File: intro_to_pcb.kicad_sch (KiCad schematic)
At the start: 0 parts

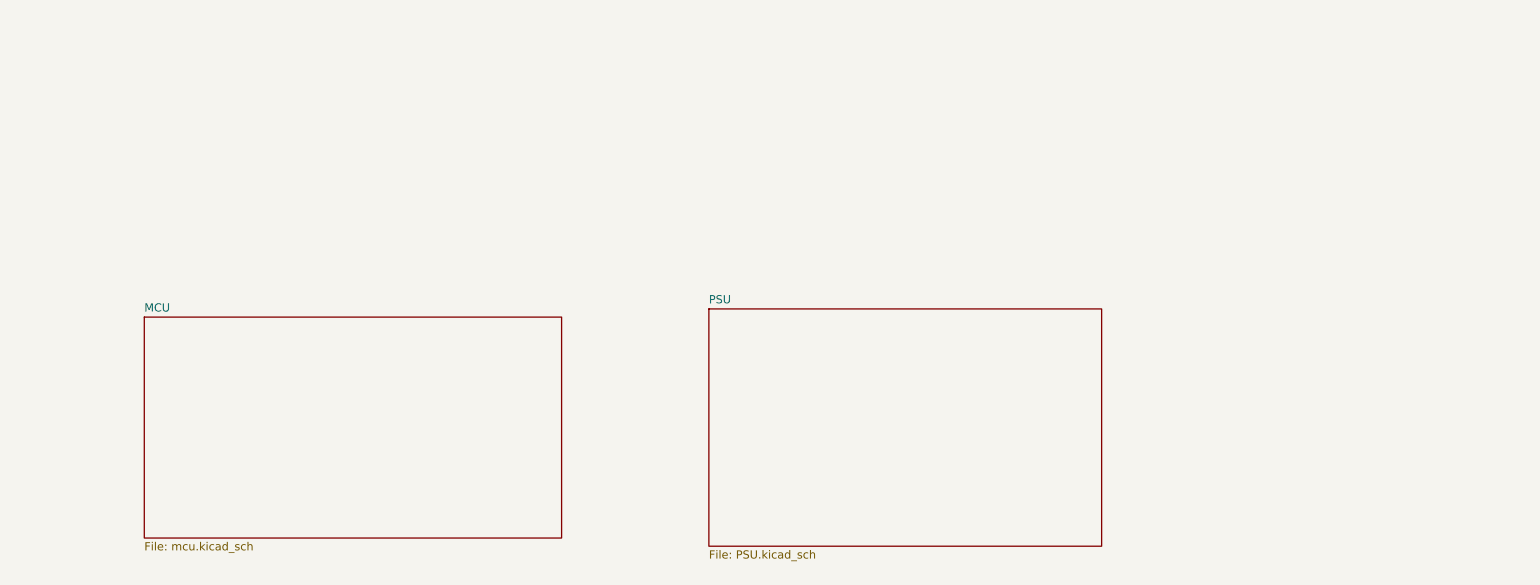
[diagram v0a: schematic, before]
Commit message: Fixing git
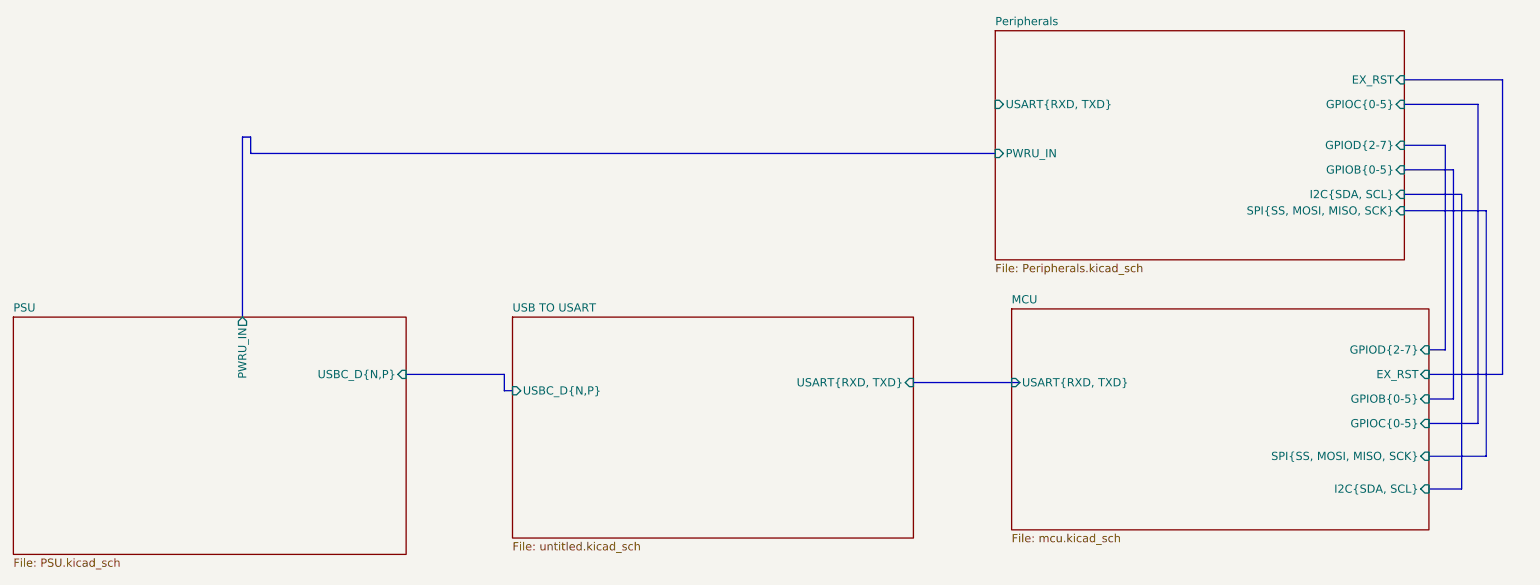
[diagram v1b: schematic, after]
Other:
- added sheet Peripherals (Peripherals.kicad_sch)
- added sheet USB TO USART (untitled.kicad_sch)
- sheet MCU ports: added EX_RST, GPIOB{0-5}, GPIOC{0-5}, GPIOD{2-7}, I2C{SDA, SCL}, SPI{SS, MOSI, MISO, SCK}, USART{RXD, TXD}; removed none
- sheet PSU ports: added PWRU_IN, USBC_D{N,P}; removed none
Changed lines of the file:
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@@
 (kicad_sch (version 20230121) (generator eeschema)
   (paper "A4")
-  (sheet (at 54.61 99.06) (size 64.77 34.29) (fields_autoplaced)
+  (bus (pts (xy 110.49 110.49) (xy 111.76 110.49))
+    (stroke (width 0) (type default))
+  )
+  (bus (pts (xy 71.12 71.12) (xy 69.85 71.12))
+    (stroke (width 0) (type default))
+  )
+  (bus (pts (xy 262.89 82.55) (xy 250.19 82.55))
+    (stroke (width 0) (type default))
+  )
+  (bus (pts (xy 257.81 111.76) (xy 254 111.76))
+    (stroke (width 0) (type default))
+  )
+  (bus (pts (xy 250.19 76.2) (xy 257.81 76.2))
+    (stroke (width 0) (type default))
+  )
+  (bus (pts (xy 265.43 107.95) (xy 254 107.95))
+    (stroke (width 0) (type default))
+  )
+  (bus (pts (xy 257.81 76.2) (xy 257.81 111.76))
+    (stroke (width 0) (type default))
+  )
+  (bus (pts (xy 110.49 107.95) (xy 110.49 110.49))
+    (stroke (width 0) (type default))
+  )
+  (bus (pts (xy 256.54 72.39) (xy 256.54 104.14))
+    (stroke (width 0) (type default))
+  )
+  (bus (pts (xy 261.62 115.57) (xy 254 115.57))
+    (stroke (width 0) (type default))
+  )
+  (bus (pts (xy 173.99 109.22) (xy 190.5 109.22))
+    (stroke (width 0) (type default))
+  )
+  (bus (pts (xy 254 125.73) (xy 259.08 125.73))
+    (stroke (width 0) (type default))
+  )
+  (bus (pts (xy 71.12 71.12) (xy 71.12 73.66))
+    (stroke (width 0) (type default))
+  )
+  (bus (pts (xy 95.25 107.95) (xy 110.49 107.95))
+    (stroke (width 0) (type default))
+  )
+  (bus (pts (xy 265.43 62.23) (xy 265.43 107.95))
+    (stroke (width 0) (type default))
+  )
+  (bus (pts (xy 262.89 120.65) (xy 262.89 82.55))
+    (stroke (width 0) (type default))
+  )
+  (bus (pts (xy 259.08 80.01) (xy 250.19 80.01))
+    (stroke (width 0) (type default))
+  )
+  (bus (pts (xy 250.19 62.23) (xy 265.43 62.23))
+    (stroke (width 0) (type default))
+  )
+  (bus (pts (xy 250.19 72.39) (xy 256.54 72.39))
+    (stroke (width 0) (type default))
+  )
+  (bus (pts (xy 259.08 125.73) (xy 259.08 80.01))
+    (stroke (width 0) (type default))
+  )
+  (bus (pts (xy 261.62 66.04) (xy 261.62 115.57))
+    (stroke (width 0) (type default))
+  )
+  (bus (pts (xy 69.85 71.12) (xy 69.85 99.06))
+    (stroke (width 0) (type default))
+  )
+  (bus (pts (xy 256.54 104.14) (xy 254 104.14))
+    (stroke (width 0) (type default))
+  )
+  (bus (pts (xy 71.12 73.66) (xy 186.69 73.66))
+    (stroke (width 0) (type default))
+  )
+  (bus (pts (xy 250.19 66.04) (xy 261.62 66.04))
+    (stroke (width 0) (type default))
+  )
+  (bus (pts (xy 254 120.65) (xy 262.89 120.65))
+    (stroke (width 0) (type default))
+  )
+  (sheet (at 111.76 99.06) (size 62.23 34.29) (fields_autoplaced)
     (stroke (width 0.1524) (type solid))
     (fill (color 0 0 0 0.0000))
-    (property "Sheetname" "MCU" (at 54.61 98.3484 0)
+    (property "Sheetname" "USB TO USART" (at 111.76 98.3484 0)
       (effects (font (size 1.27 1.27)) (justify left bottom))
     )
-    (property "Sheetfile" "mcu.kicad_sch" (at 54.61 133.9346 0)
+    (property "Sheetfile" "untitled.kicad_sch" (at 111.76 133.9346 0)
       (effects (font (size 1.27 1.27)) (justify left top))
+    )
+    (pin "USBC_D{N,P}" input (at 111.76 110.49 180)
+      (effects (font (size 1.27 1.27)) (justify left))
+    )
+    (pin "USART{RXD, TXD}" input (at 173.99 109.22 0)
+      (effects (font (size 1.27 1.27)) (justify right))
+    )
+    (instances
+      (project "intro_to_pcb"
+        (path "/b2bbdadf-112f-4546-9689-8793d1774710" (page "4"))
+      )
+    )
+  )
+  (sheet (at 189.23 97.79) (size 64.77 34.29) (fields_autoplaced)
+    (stroke (width 0.1524) (type solid))
+    (fill (color 0 0 0 0.0000))
+    (property "Sheetname" "MCU" (at 189.23 97.0784 0)
+      (effects (font (size 1.27 1.27)) (justify left bottom))
+    )
+    (property "Sheetfile" "mcu.kicad_sch" (at 189.23 132.6646 0)
+      (effects (font (size 1.27 1.27)) (justify left top))
+    )
+    (pin "GPIOD{2-7}" input (at 254 104.14 0)
+      (effects (font (size 1.27 1.27)) (justify right))
+    )
+    (pin "EX_RST" input (at 254 107.95 0)
+      (effects (font (size 1.27 1.27)) (justify right))
+    )
+    (pin "GPIOB{0-5}" input (at 254 111.76 0)
+      (effects (font (size 1.27 1.27)) (justify right))
+    )
+    (pin "GPIOC{0-5}" input (at 254 115.57 0)
+      (effects (font (size 1.27 1.27)) (justify right))
+    )
+    (pin "SPI{SS, MOSI, MISO, SCK}" input (at 254 120.65 0)
+      (effects (font (size 1.27 1.27)) (justify right))
+    )
+    (pin "USART{RXD, TXD}" input (at 189.23 109.22 180)
+      (effects (font (size 1.27 1.27)) (justify left))
+    )
+    (pin "I2C{SDA, SCL}" input (at 254 125.73 0)
+      (effects (font (size 1.27 1.27)) (justify right))
     )
     (instances
@@
     )
   )
-  (sheet (at 142.24 97.79) (size 60.96 36.83) (fields_autoplaced)
+  (sheet (at 186.69 54.61) (size 63.5 35.56) (fields_autoplaced)
     (stroke (width 0.1524) (type solid))
     (fill (color 0 0 0 0.0000))
-    (property "Sheetname" "PSU" (at 142.24 97.0784 0)
+    (property "Sheetname" "Peripherals" (at 186.69 53.8984 0)
       (effects (font (size 1.27 1.27)) (justify left bottom))
     )
-    (property "Sheetfile" "PSU.kicad_sch" (at 142.24 135.2046 0)
+    (property "Sheetfile" "Peripherals.kicad_sch" (at 186.69 90.7546 0)
       (effects (font (size 1.27 1.27)) (justify left top))
     )
+    (pin "EX_RST" input (at 250.19 62.23 0)
+      (effects (font (size 1.27 1.27)) (justify right))
+    )
+    (pin "GPIOC{0-5}" input (at 250.19 66.04 0)
+      (effects (font (size 1.27 1.27)) (justify right))
+    )
+    (pin "GPIOD{2-7}" input (at 250.19 72.39 0)
+      (effects (font (size 1.27 1.27)) (justify right))
+    )
+    (pin "GPIOB{0-5}" input (at 250.19 76.2 0)
+      (effects (font (size 1.27 1.27)) (justify right))
+    )
+    (pin "SPI{SS, MOSI, MISO, SCK}" input (at 250.19 82.55 0)
+      (effects (font (size 1.27 1.27)) (justify right))
+    )
+    (pin "USART{RXD, TXD}" input (at 186.69 66.04 180)
+      (effects (font (size 1.27 1.27)) (justify left))
+    )
+    (pin "I2C{SDA, SCL}" input (at 250.19 80.01 0)
+      (effects (font (size 1.27 1.27)) (justify right))
+    )
+    (pin "PWRU_IN" input (at 186.69 73.66 180)
+      (effects (font (size 1.27 1.27)) (justify left))
+    )
     (instances
+      (project "intro_to_pcb"
+        (path "/b2bbdadf-112f-4546-9689-8793d1774710" (page "5"))
+      )
+    )
+  )
+  (sheet (at 34.29 99.06) (size 60.96 36.83) (fields_autoplaced)
+    (stroke (width 0.1524) (type solid))
+    (fill (color 0 0 0 0.0000))
+    (property "Sheetname" "PSU" (at 34.29 98.3484 0)
+      (effects (font (size 1.27 1.27)) (justify left bottom))
+    )
+    (property "Sheetfile" "PSU.kicad_sch" (at 34.29 136.4746 0)
+      (effects (font (size 1.27 1.27)) (justify left top))
+    )
+    (pin "USBC_D{N,P}" input (at 95.25 107.95 0)
+      (effects (font (size 1.27 1.27)) (justify right))
+    )
+    (pin "PWRU_IN" output (at 69.85 99.06 90)
+      (effects (font (size 1.27 1.27)) (justify right))
+    )
+    (instances

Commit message: updated
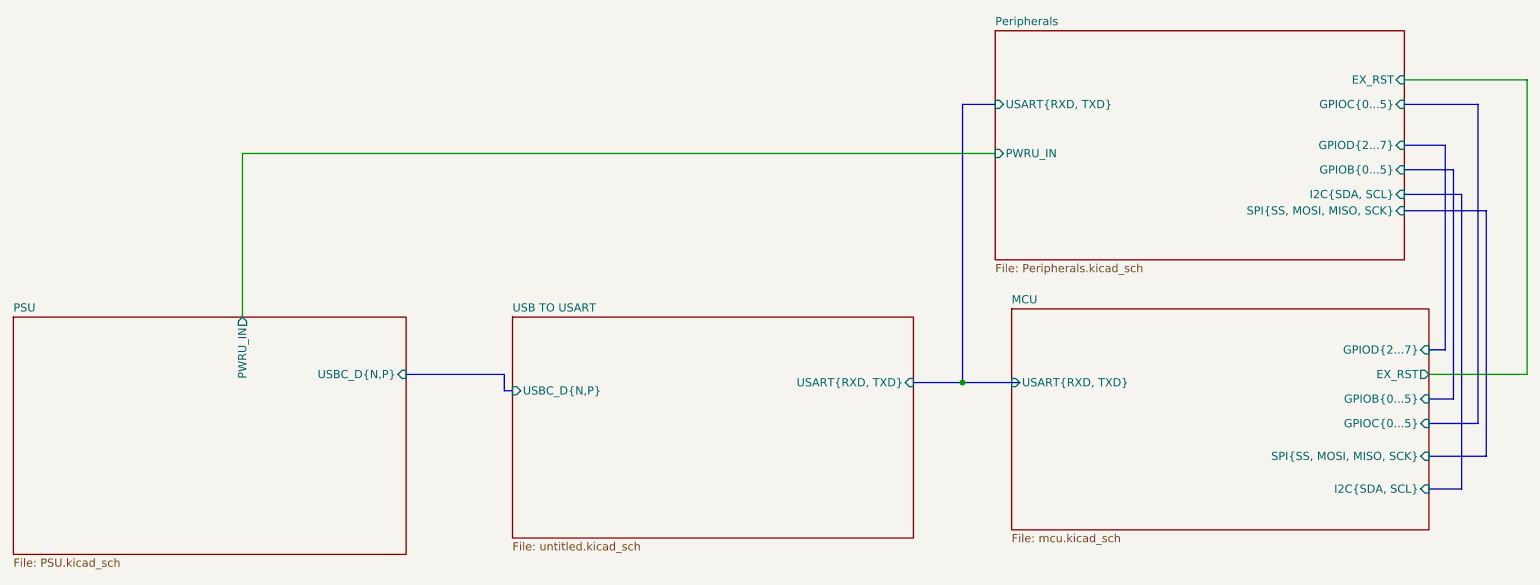
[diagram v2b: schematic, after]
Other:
- sheet MCU ports: added GPIOB{0...5}, GPIOC{0...5}, GPIOD{2...7}; removed GPIOB{0-5}, GPIOC{0-5}, GPIOD{2-7}
- sheet Peripherals ports: added GPIOB{0...5}, GPIOC{0...5}, GPIOD{2...7}; removed GPIOB{0-5}, GPIOC{0-5}, GPIOD{2-7}
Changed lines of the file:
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@@
 (kicad_sch (version 20230121) (generator eeschema)
   (paper "A4")
+  (junction (at 181.61 109.22) (diameter 0) (color 0 0 0 0)
+  )
   (bus (pts (xy 110.49 110.49) (xy 111.76 110.49))
-    (stroke (width 0) (type default))
-  )
-  (bus (pts (xy 71.12 71.12) (xy 69.85 71.12))
     (stroke (width 0) (type default))
   )
@@
     (stroke (width 0) (type default))
   )
-  (bus (pts (xy 265.43 107.95) (xy 254 107.95))
+  (wire (pts (xy 250.19 62.23) (xy 269.24 62.23))
+    (stroke (width 0) (type default))
+  )
+  (bus (pts (xy 181.61 109.22) (xy 190.5 109.22))
     (stroke (width 0) (type default))
   )
@@
     (stroke (width 0) (type default))
   )
-  (bus (pts (xy 173.99 109.22) (xy 190.5 109.22))
+  (wire (pts (xy 69.85 73.66) (xy 186.69 73.66))
+    (stroke (width 0) (type default))
+  )
+  (bus (pts (xy 173.99 109.22) (xy 181.61 109.22))
+    (stroke (width 0) (type default))
+  )
+  (wire (pts (xy 269.24 107.95) (xy 254 107.95))
     (stroke (width 0) (type default))
   )
@@
     (stroke (width 0) (type default))
   )
-  (bus (pts (xy 71.12 71.12) (xy 71.12 73.66))
-    (stroke (width 0) (type default))
-  )
   (bus (pts (xy 95.25 107.95) (xy 110.49 107.95))
     (stroke (width 0) (type default))
   )
-  (bus (pts (xy 265.43 62.23) (xy 265.43 107.95))
+  (bus (pts (xy 186.69 66.04) (xy 181.61 66.04))
+    (stroke (width 0) (type default))
+  )
+  (wire (pts (xy 69.85 99.06) (xy 69.85 73.66))
     (stroke (width 0) (type default))
   )
@@
     (stroke (width 0) (type default))
   )
-  (bus (pts (xy 250.19 62.23) (xy 265.43 62.23))
+  (bus (pts (xy 250.19 72.39) (xy 256.54 72.39))
     (stroke (width 0) (type default))
   )
-  (bus (pts (xy 250.19 72.39) (xy 256.54 72.39))
+  (bus (pts (xy 181.61 66.04) (xy 181.61 109.22))
     (stroke (width 0) (type default))
   )
@@
     (stroke (width 0) (type default))
   )
-  (bus (pts (xy 69.85 71.12) (xy 69.85 99.06))
+  (wire (pts (xy 269.24 62.23) (xy 269.24 107.95))
     (stroke (width 0) (type default))
   )
   (bus (pts (xy 256.54 104.14) (xy 254 104.14))
-    (stroke (width 0) (type default))
-  )
-  (bus (pts (xy 71.12 73.66) (xy 186.69 73.66))
     (stroke (width 0) (type default))
   )
@@
       (effects (font (size 1.27 1.27)) (justify left top))
     )
-    (pin "GPIOD{2-7}" input (at 254 104.14 0)
-      (effects (font (size 1.27 1.27)) (justify right))
-    )
-    (pin "EX_RST" input (at 254 107.95 0)
-      (effects (font (size 1.27 1.27)) (justify right))
-    )
-    (pin "GPIOB{0-5}" input (at 254 111.76 0)
-      (effects (font (size 1.27 1.27)) (justify right))
-    )
-    (pin "GPIOC{0-5}" input (at 254 115.57 0)
+    (pin "EX_RST" output (at 254 107.95 0)
       (effects (font (size 1.27 1.27)) (justify right))
     )
@@
     )
     (pin "I2C{SDA, SCL}" input (at 254 125.73 0)
+      (effects (font (size 1.27 1.27)) (justify right))
+    )
+    (pin "GPIOC{0...5}" input (at 254 115.57 0)
+      (effects (font (size 1.27 1.27)) (justify right))
+    )
+    (pin "GPIOB{0...5}" input (at 254 111.76 0)
+      (effects (font (size 1.27 1.27)) (justify right))
+    )
+    (pin "GPIOD{2...7}" input (at 254 104.14 0)
       (effects (font (size 1.27 1.27)) (justify right))
     )
@@
       (effects (font (size 1.27 1.27)) (justify right))
     )
-    (pin "GPIOC{0-5}" input (at 250.19 66.04 0)
-      (effects (font (size 1.27 1.27)) (justify right))
-    )
-    (pin "GPIOD{2-7}" input (at 250.19 72.39 0)
-      (effects (font (size 1.27 1.27)) (justify right))
-    )
-    (pin "GPIOB{0-5}" input (at 250.19 76.2 0)
-      (effects (font (size 1.27 1.27)) (justify right))
-    )
     (pin "SPI{SS, MOSI, MISO, SCK}" input (at 250.19 82.55 0)
       (effects (font (size 1.27 1.27)) (justify right))
@@
       (effects (font (size 1.27 1.27)) (justify left))
     )
+    (pin "GPIOC{0...5}" input (at 250.19 66.04 0)
+      (effects (font (size 1.27 1.27)) (justify right))
+    )
+    (pin "GPIOD{2...7}" input (at 250.19 72.39 0)
+      (effects (font (size 1.27 1.27)) (justify right))
+    )
+    (pin "GPIOB{0...5}" input (at 250.19 76.2 0)
+      (effects (font (size 1.27 1.27)) (justify right))
+    )
     (instances
